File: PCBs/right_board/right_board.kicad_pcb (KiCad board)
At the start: 2 copper layers, 143.8 x 139.6 mm, 104 parts, among them J101 USB4510-03-1-A, J102 Conn_ARM_SWD_TagConnect_TC2030, J103 GSB12J21C1EU, J104 USB4510-03-1-A, SW101 SW_DIP_x01, SW102 SW_DIP_x01, SW103 SW_DIP_x01, SW104 SW_DIP_x01, SW105 SW_DIP_x01, SW106 SW_DIP_x01, SW107 SW_DIP_x01, SW108 SW_DIP_x01, SW109 SW_DIP_x01, SW110 SW_DIP_x01, SW111 SW_DIP_x01, SW112 SW_DIP_x01, SW113 SW_DIP_x01, SW114 SW_DIP_x01, SW115 SW_DIP_x01, SW116 SW_DIP_x01, SW117 SW_DIP_x01, SW118 SW_DIP_x01, SW119 SW_DIP_x01, SW120 SW_DIP_x01, SW121 SW_DIP_x01, SW122 SW_DIP_x01, SW123 SW_DIP_x01, SW124 SW_DIP_x01, SW125 SW_DIP_x01, SW126 SW_DIP_x01, SW127 SW_DIP_x01, SW128 RIC11-31S15.5D7-TH, U101 STM32G0C1CEUx, U102 USB2533-1080AEN, U103 M24256X-FCU6T_VF, U104 USBLC6-4SC6, U105 USBLC6-4SC6, U106 USBLC6-4SC6, Y101 CX2016SA24000D0HLLG3

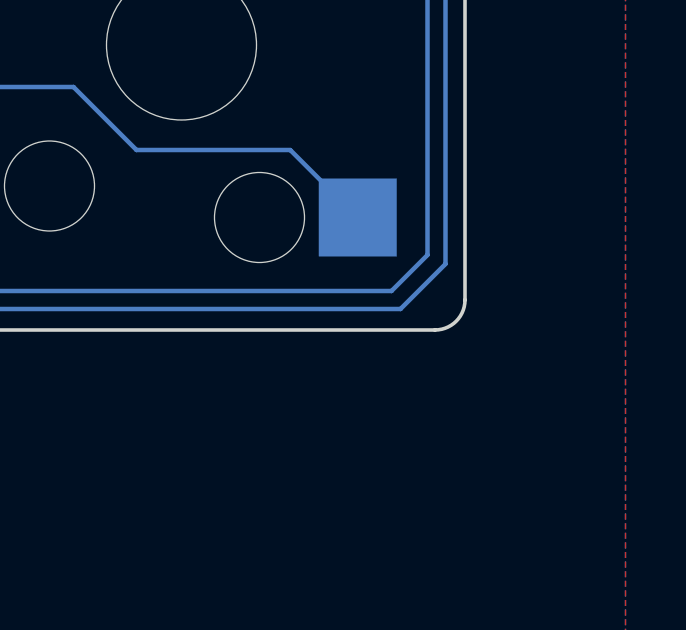
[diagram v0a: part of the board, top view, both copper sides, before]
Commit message: Pinout updates
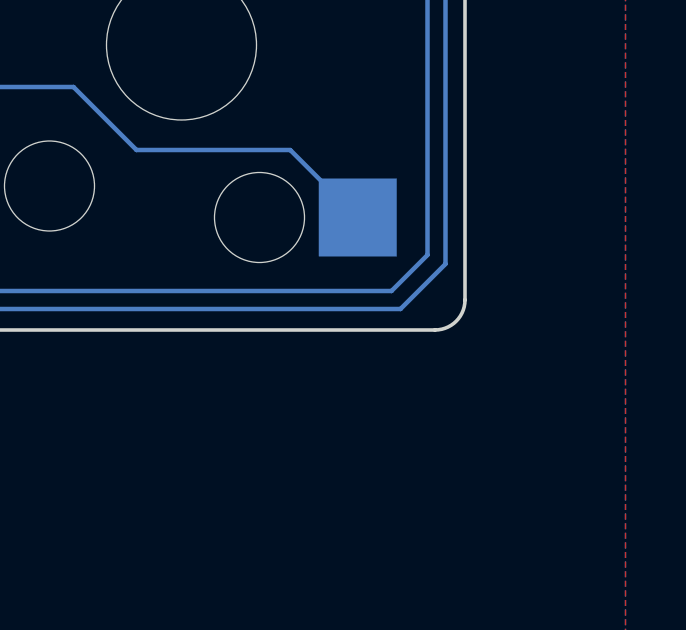
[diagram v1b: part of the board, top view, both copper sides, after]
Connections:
- net /KEY_A1 renamed /KEY_A7
- net /KEY_A2 renamed /KEY_A8
- net /KEY_A3 renamed /KEY_A9
- net /KEY_A4 renamed /KEY_A10
- net /KEY_A5 renamed /KEY_A11
- net /KEY_A6 renamed /KEY_A12
- net /KEY_B1 renamed /KEY_B7
- net /KEY_B2 renamed /KEY_B8
- net /KEY_B3 renamed /KEY_B9
- net /KEY_B4 renamed /KEY_B10
- net /KEY_B5 renamed /KEY_B11
- net /KEY_B6 renamed /KEY_B12
- net /KEY_C1 renamed /KEY_C7
- net /KEY_C2 renamed /KEY_C8
- net /KEY_C3 renamed /KEY_C9
- net /KEY_C4 renamed /KEY_C10
- net /KEY_C5 renamed /KEY_C11
- net /KEY_C6 renamed /KEY_C12
- net /KEY_D1 renamed /KEY_D7
- net /KEY_D2 renamed /KEY_D8
- net /KEY_D3 renamed /KEY_D9
- net /KEY_D4 renamed /KEY_D10
- net /KEY_D5 renamed /KEY_D11
- net /KEY_D6 renamed /KEY_D12
- net /KEY_E1 renamed /KEY_E6
- net /KEY_E2 renamed /KEY_E5
- net /KEY_E3 renamed /KEY_E4
